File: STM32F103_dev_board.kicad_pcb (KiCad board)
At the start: 4 copper layers, 39.4 x 83.8 mm, 37 parts, among them IC1 TLV70233DBVR, IC2 FT232RNL-REEL, J1 Conn_ARM_JTAG_SWD_20, J2 Conn_01x20_Pin, J3 Conn_01x20_Pin, J4 Conn_02x03_Odd_Even, J6 USB4800-03-A, U1 STM32F103RBTx, Y1 8MHz, Y2 Crystal_GND23

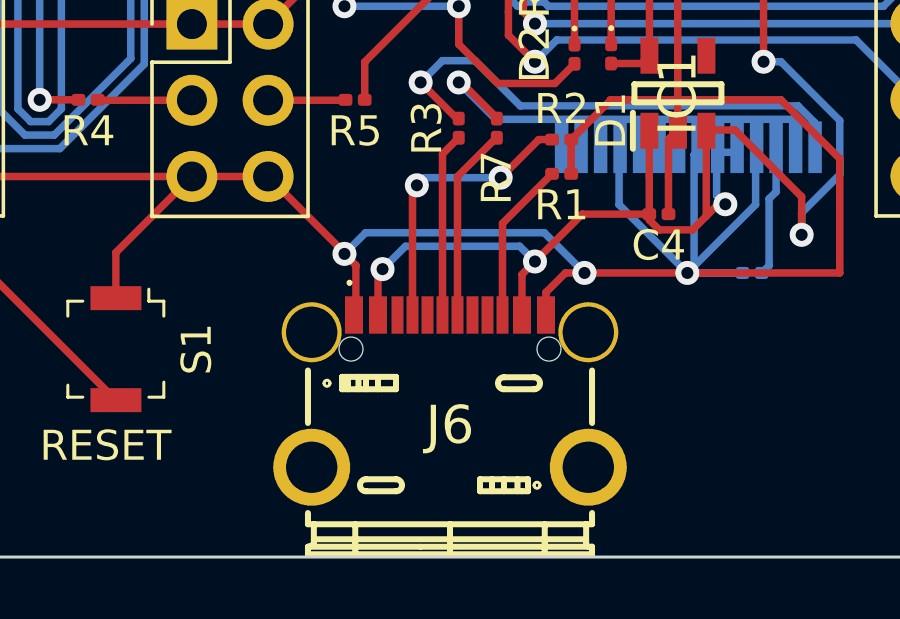
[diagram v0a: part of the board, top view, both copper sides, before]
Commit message: Updated production files
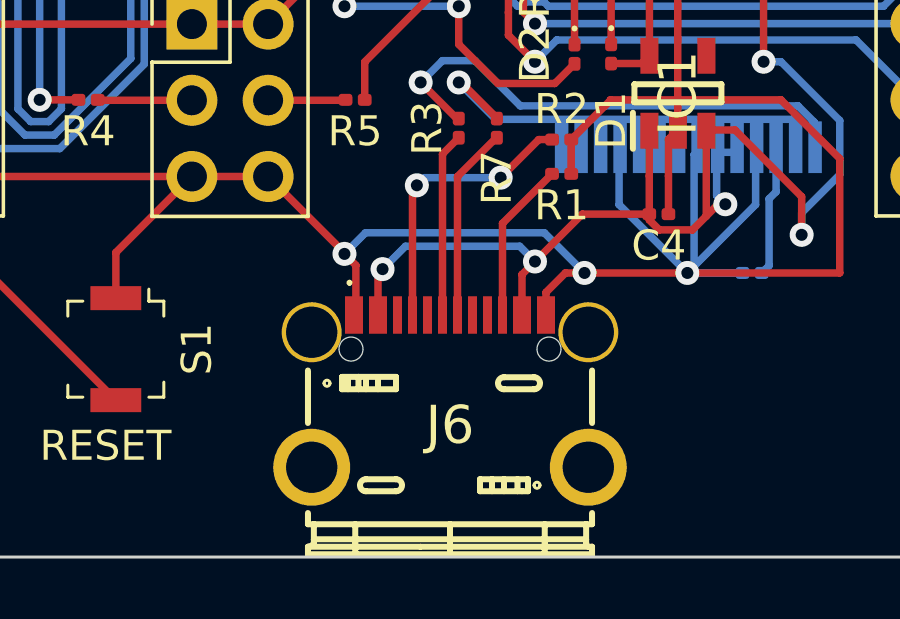
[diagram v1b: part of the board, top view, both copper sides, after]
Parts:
- J6: footprint SamacSys_Parts:USB480003A_BIGPAD -> SamacSys_Parts:USB480003A
